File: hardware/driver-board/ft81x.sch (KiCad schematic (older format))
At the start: 7 parts, among them U6 FT813, X1 YSX321SL

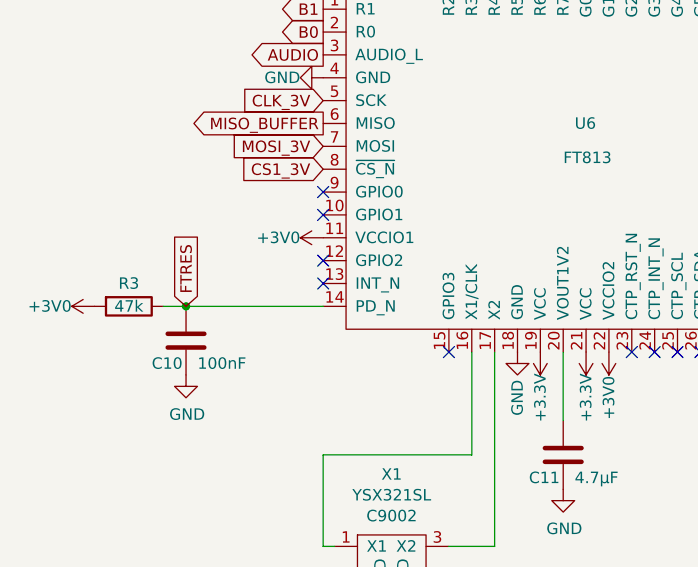
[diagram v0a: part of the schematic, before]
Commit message: Board layout on work
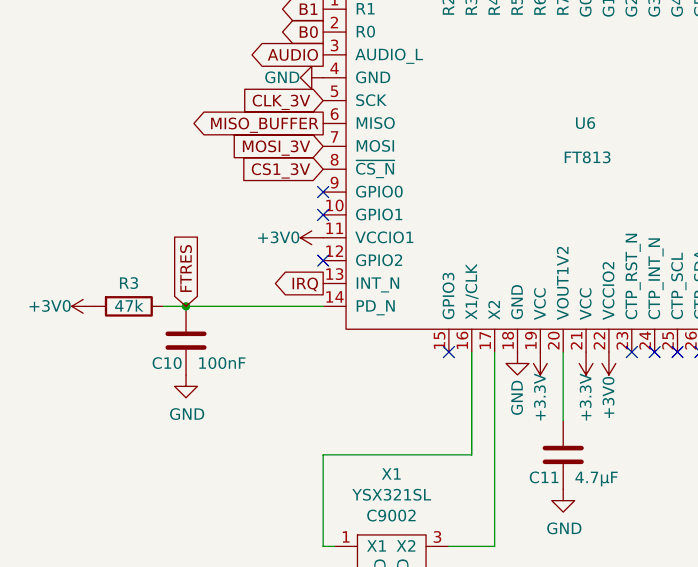
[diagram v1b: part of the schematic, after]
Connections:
- net IRQ: now reaches U6.13 (INT_N)
- no-connect marks 11 -> 10
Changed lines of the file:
@@
 NoConn ~ 7100 2600
 NoConn ~ 5300 3100
-NoConn ~ 4750 2800
 NoConn ~ 4750 2700
 NoConn ~ 4750 2500
@@
 Text GLabel 4150 2900 1    50   Input ~ 0
 FTRES
+Text GLabel 4750 2800 0    50   Output ~ 0
+IRQ
 $EndSCHEMATC
